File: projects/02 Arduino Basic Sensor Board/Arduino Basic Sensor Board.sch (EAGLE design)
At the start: 47 parts, among them Q1 S8050SOT23, Q2 S8050SOT23

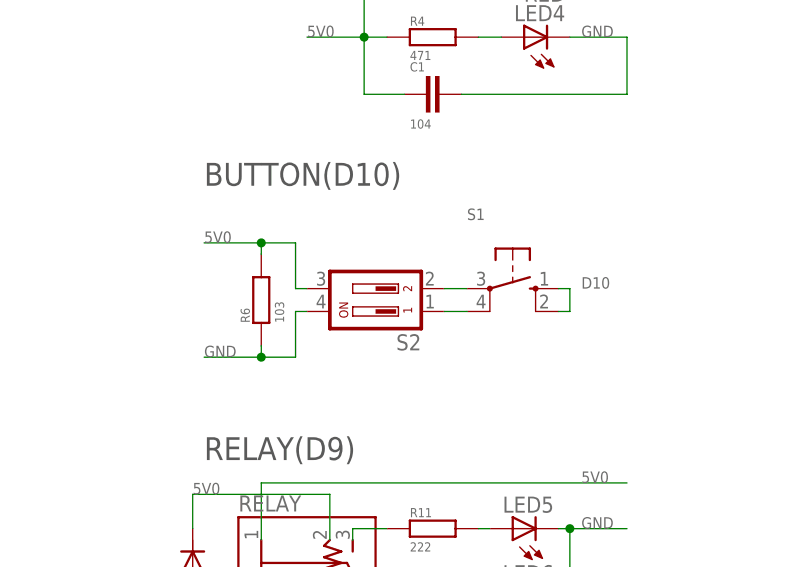
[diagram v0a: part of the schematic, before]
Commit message: 2020.06.22.01
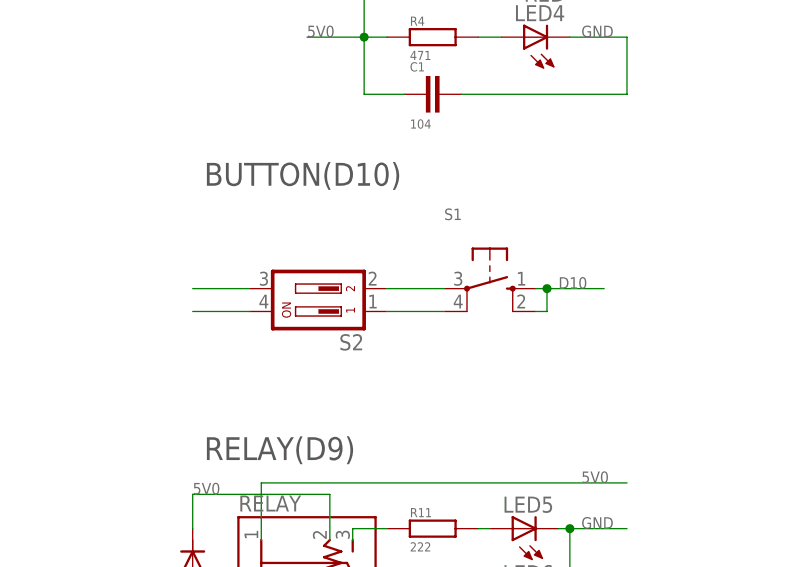
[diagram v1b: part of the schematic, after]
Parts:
- removed R6: 103, RCLDA:R0805
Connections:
- new net N$16: S2.3
- new net N$17: S2.4
- net 5V0: no longer R6.2, S2.3
- net GND: no longer R6.1, S2.4
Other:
- moved on the sheet: S1, S2
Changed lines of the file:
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@@
 <setting verticaltext="up"/>
 </settings>
-<grid distance="0.1" unitdist="inch" unit="inch" style="lines" multiple="1" display="no" altdistance="0.01" altunitdist="inch" altunit="inch"/>
+<grid distance="50" unitdist="mil" unit="mil" style="lines" multiple="1" display="yes" altdistance="25" altunitdist="mil" altunit="mil"/>
 <layers>
 <layer number="1" name="Top" color="4" fill="1" visible="no" active="no"/>
@@
 <part name="FRAME1" library="Frame" deviceset="A4-H" device=""/>
 <part name="U$1" library="Module" deviceset="ARDUINO-UNO" device="" value=""/>
-<part name="S1" library="Button" deviceset="TS-DIP-4.5*4.5" device=""/>
-<part name="S2" library="Switch" deviceset="SD4-02" device=""/>
 <part name="LED4" library="Display" deviceset="LED" device="CHIPLED_0805" value="RED"/>
 <part name="U$2" library="Senser" deviceset="3362" device="3362" value=""/>
@@
 <part name="Q1" library="RCLDA" deviceset="S8050" device="SOT23" value=""/>
 <part name="Q2" library="RCLDA" deviceset="S8050" device="SOT23" value=""/>
-<part name="R6" library="RCLDA" deviceset="R" device="0805" value="103"/>
 <part name="R7" library="RCLDA" deviceset="R" device="0805" value="222"/>
 <part name="D1" library="RCLDA" deviceset="DIODE" device="SMB" value=""/>
@@
 <part name="LED3" library="Display" deviceset="LED" device="CHIPLED_0805" value="RED"/>
 <part name="GND3" library="Power" deviceset="GND" device=""/>
+<part name="S1" library="Button" deviceset="TS-DIP-4.5*4.5" device=""/>
+<part name="S2" library="Switch" deviceset="SD4-02" device=""/>
 </parts>
 <sheets>
@@
 <instance part="FRAME1" gate="G$1" x="0" y="0"/>
 <instance part="U$1" gate="G$1" x="53.34" y="148.59"/>
-<instance part="S1" gate="1" x="64.77" y="59.69"/>
-<instance part="S2" gate="1" x="49.53" y="57.15" rot="R90"/>
 <instance part="LED4" gate="G$1" x="66.04" y="87.63" rot="R90"/>
 <instance part="U$2" gate="G$1" x="227.33" y="121.92"/>
@@
 <instance part="Q1" gate="G$1" x="26.67" y="16.51"/>
 <instance part="Q2" gate="G$1" x="120.65" y="144.78"/>
-<instance part="R6" gate="G$1" x="36.83" y="58.42" rot="R90"/>
 <instance part="R7" gate="G$1" x="17.78" y="16.51"/>
 <instance part="D1" gate="G$1" x="29.21" y="29.21" rot="R90"/>
@@
 <instance part="LED3" gate="G$1" x="182.88" y="106.68" rot="R90"/>
 <instance part="GND3" gate="1" x="193.04" y="106.68" rot="R90"/>
+<instance part="S1" gate="1" x="62.23" y="59.69"/>
+<instance part="S2" gate="1" x="43.18" y="57.15" rot="R90"/>
 </instances>
 <busses>
@@
 <segment>
 <pinref part="S1" gate="1" pin="S"/>
-<wire x1="69.85" y1="59.69" x2="71.12" y2="59.69" width="0.1524" layer="91"/>
-<wire x1="71.12" y1="59.69" x2="71.12" y2="57.15" width="0.1524" layer="91"/>
+<wire x1="67.31" y1="59.69" x2="68.58" y2="59.69" width="0.1524" layer="91"/>
+<wire x1="68.58" y1="59.69" x2="68.58" y2="57.15" width="0.1524" layer="91"/>
 <pinref part="S1" gate="1" pin="S1"/>
-<wire x1="71.12" y1="57.15" x2="69.85" y2="57.15" width="0.1524" layer="91"/>
-<label x="72.39" y="59.69" size="1.27" layer="95"/>
+<wire x1="68.58" y1="57.15" x2="67.31" y2="57.15" width="0.1524" layer="91"/>
+<wire x1="74.93" y1="59.69" x2="68.58" y2="59.69" width="0.1524" layer="91"/>
+<junction x="68.58" y="59.69"/>
+<label x="69.85" y="59.69" size="1.27" layer="95"/>
 </segment>
 </net>
@@
 <wire x1="77.47" y1="81.28" x2="77.47" y2="87.63" width="0.1524" layer="91"/>
 <pinref part="C1" gate="G$1" pin="1"/>
-</segment>
-<segment>
-<pinref part="S2" gate="1" pin="4"/>
-<wire x1="41.91" y1="57.15" x2="40.64" y2="57.15" width="0.1524" layer="91"/>
-<wire x1="40.64" y1="57.15" x2="40.64" y2="52.07" width="0.1524" layer="91"/>
-<wire x1="40.64" y1="52.07" x2="36.83" y2="52.07" width="0.1524" layer="91"/>
-<pinref part="R6" gate="G$1" pin="1"/>
-<wire x1="36.83" y1="52.07" x2="30.48" y2="52.07" width="0.1524" layer="91"/>
-<wire x1="36.83" y1="53.34" x2="36.83" y2="52.07" width="0.1524" layer="91"/>
-<junction x="36.83" y="52.07"/>
-<label x="30.48" y="52.07" size="1.27" layer="95"/>
 </segment>
 <segment>
@@
 </segment>
 <segment>
-<pinref part="S2" gate="1" pin="3"/>
-<wire x1="41.91" y1="59.69" x2="40.64" y2="59.69" width="0.1524" layer="91"/>
-<wire x1="40.64" y1="59.69" x2="40.64" y2="64.77" width="0.1524" layer="91"/>
-<wire x1="40.64" y1="64.77" x2="36.83" y2="64.77" width="0.1524" layer="91"/>
-<pinref part="R6" gate="G$1" pin="2"/>
-<wire x1="36.83" y1="64.77" x2="30.48" y2="64.77" width="0.1524" layer="91"/>
-<wire x1="36.83" y1="63.5" x2="36.83" y2="64.77" width="0.1524" layer="91"/>
-<junction x="36.83" y="64.77"/>
-<label x="30.48" y="64.77" size="1.27" layer="95"/>
-</segment>
-<segment>
 <pinref part="U$6" gate="G$1" pin="P$1"/>
 <wire x1="215.265" y1="154.94" x2="208.915" y2="154.94" width="0.1524" layer="91"/>
@@
 </segment>
 </net>
-<net name="N$5" class="0">
-<segment>
-<pinref part="S1" gate="1" pin="P1"/>
-<pinref part="S2" gate="1" pin="1"/>
-<wire x1="57.15" y1="57.15" x2="59.69" y2="57.15" width="0.1524" layer="91"/>
-</segment>
-</net>
-<net name="N$6" class="0">
-<segment>
-<pinref part="S1" gate="1" pin="P"/>
-<pinref part="S2" gate="1" pin="2"/>
-<wire x1="57.15" y1="59.69" x2="59.69" y2="59.69" width="0.1524" layer="91"/>
-</segment>
-</net>
 <net name="N$32" class="0">
 <segment>
@@
 </segment>
 </net>
+<net name="N$5" class="0">
+<segment>
+<pinref part="S1" gate="1" pin="P1"/>
+<pinref part="S2" gate="1" pin="1"/>
+<wire x1="50.8" y1="57.15" x2="57.15" y2="57.15" width="0.1524" layer="91"/>
+</segment>
+</net>
+<net name="N$6" class="0">
+<segment>
+<pinref part="S1" gate="1" pin="P"/>
+<pinref part="S2" gate="1" pin="2"/>
+<wire x1="50.8" y1="59.69" x2="57.15" y2="59.69" width="0.1524" layer="91"/>
+</segment>
+</net>
+<net name="N$16" class="0">
+<segment>
+<pinref part="S2" gate="1" pin="3"/>
+<wire x1="29.21" y1="59.69" x2="35.56" y2="59.69" width="0.1524" layer="91"/>
+</segment>
+</net>
+<net name="N$17" class="0">
+<segment>
+<pinref part="S2" gate="1" pin="4"/>
+<wire x1="29.21" y1="57.15" x2="35.56" y2="57.15" width="0.1524" layer="91"/>
+</segment>
+</net>
